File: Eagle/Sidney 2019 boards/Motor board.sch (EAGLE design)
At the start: 27 parts, among them IC1 LM2596S, IC2 LM2940CS-5.0_NOPB, J1 TWIG_2.0, J2 TWIG_2.0, J3 TWIG_2.0, J4 TWIG_2.0

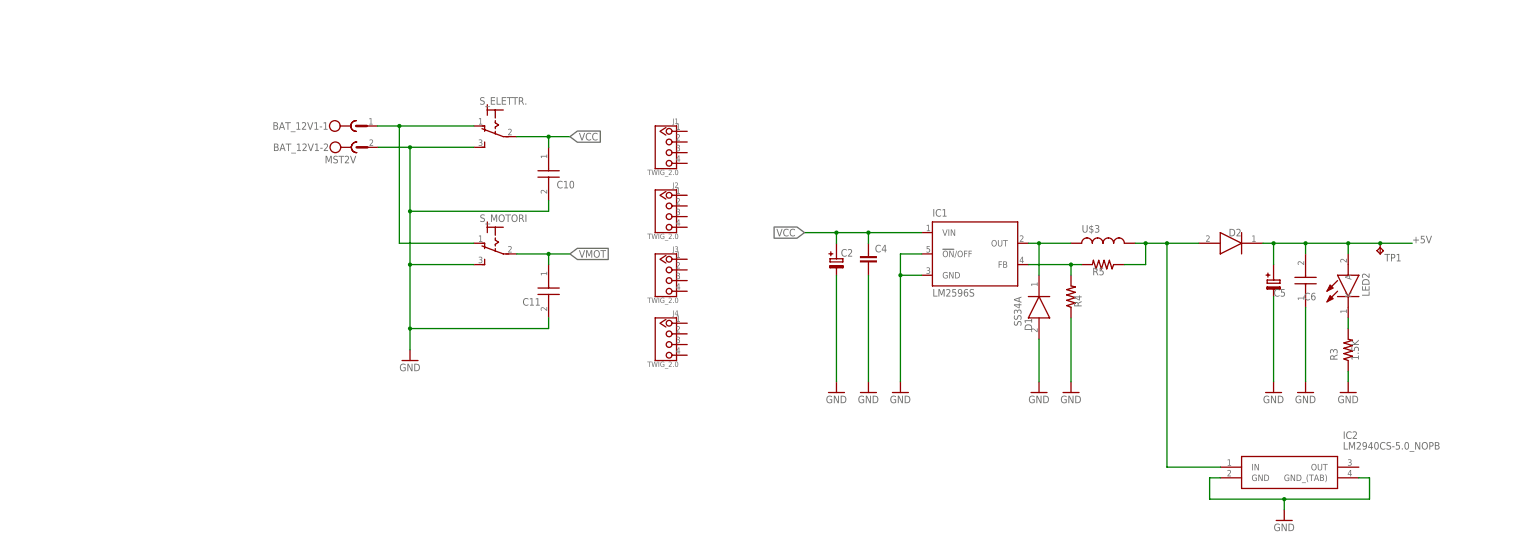
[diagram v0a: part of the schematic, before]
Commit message: general improvements to the boards
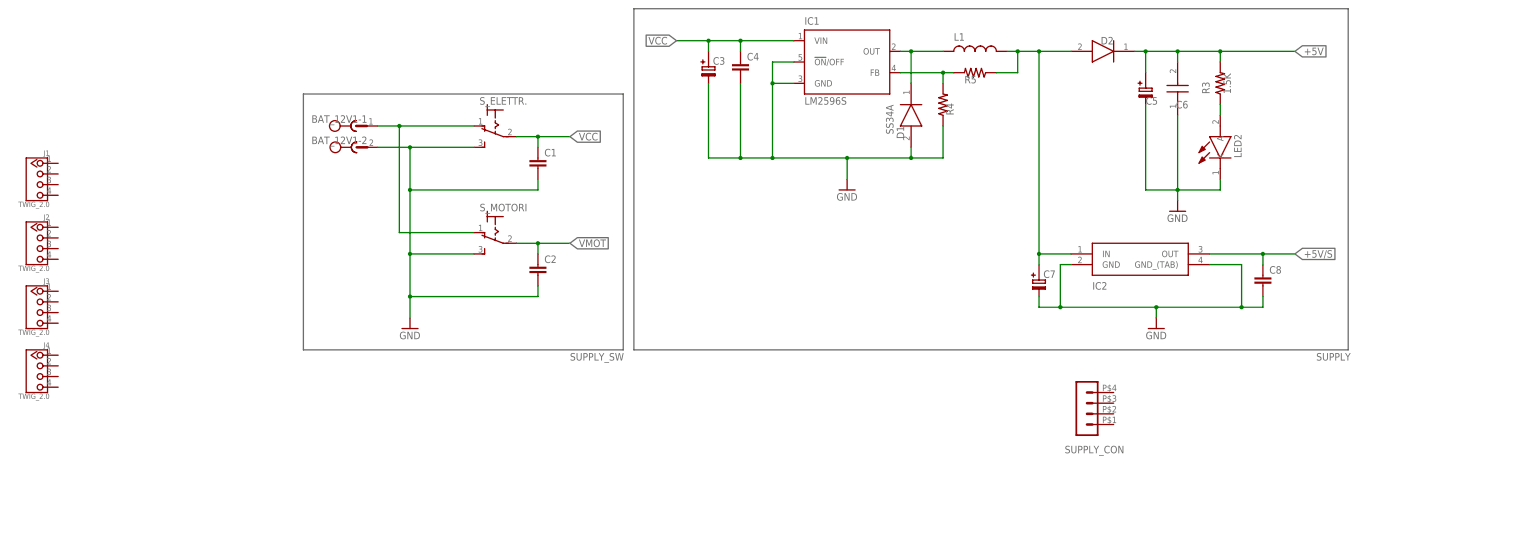
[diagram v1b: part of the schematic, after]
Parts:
- removed C10, C11: 12065D106KAT2A, 12065D106KAT2A:12065D106KAT2A
- removed TP1: TPTP13SQ, testpad:TPTP13SQ
- removed U$3: (no value), inductor-coilcraft:MSS1260
- added C1: (no value), rcl:C-EUC1206
- added C3, C7: (no value), cap-pan40:C-PR-SMD-SV-E/F
- added C8: (no value), eagle-ltspice:CC1206
- added L1: 47/470uH (?), inductor-coilcraft:MSS1260
- added SUPPLY_CON: (no value), con-molex-micro-fit-3_0:HEADER_POS4_43045-0412
- C2: device cap-pan40:C-PR-SMD-SV-E/F -> rcl:C-EUC1206
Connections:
- removed net N$8: LED2.K, R3.2
- new net +5V/S: C8.1, IC2.OUT
- new net N$3: LED2.A, R3.1
- net +5V: now also R3.2; no longer LED2.A, TP1.TP
- net 5.7V-DIRAMAZIONE2: now also C7.+, L1.P$1; no longer U$3.P$1
- net GND: now also C1.2, C2.2, C3.-, C7.-, C8.2, LED2.K; no longer C10.2, C11.2, C2.-, R3.1
- net N$6: now also L1.P$2; no longer U$3.P$2
- net VCC: now also C1.1, C3.+; no longer C10.1, C2.+
- net VMOT: now also C2.1; no longer C11.1
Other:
- note added: "SUPPLY"
- note added: "SUPPLY_SW"
- moved on the sheet: C4, C5, C6, D1, D2, IC1, IC2, J1, J2, J3, J4, LED2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
